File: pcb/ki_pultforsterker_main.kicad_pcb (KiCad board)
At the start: 2 copper layers, 150 x 100 mm, 145 parts, among them J1 24V IN, J10 LED-RINGER, J2 SPK L, J3 SPK R, J4 AUX, J5 RPi 40-pin, J6 5V -> PI, J7 KNAPPER, J8 ENCODER, J9 OLED, K1 G6K-2P-Y 5VDC, Q1 AO3400A, Q2 AO3400A, Q3 AO3400A, Q4 AO3400A, Q5 AO3400A, Q6 AO3400A, U1 TPS54560BDDA, U2 AMS1117-3.3, U3 ICL7660, U4 PCM5102APW, U5 PGA2311UA, U6 TPA3116D2DAD

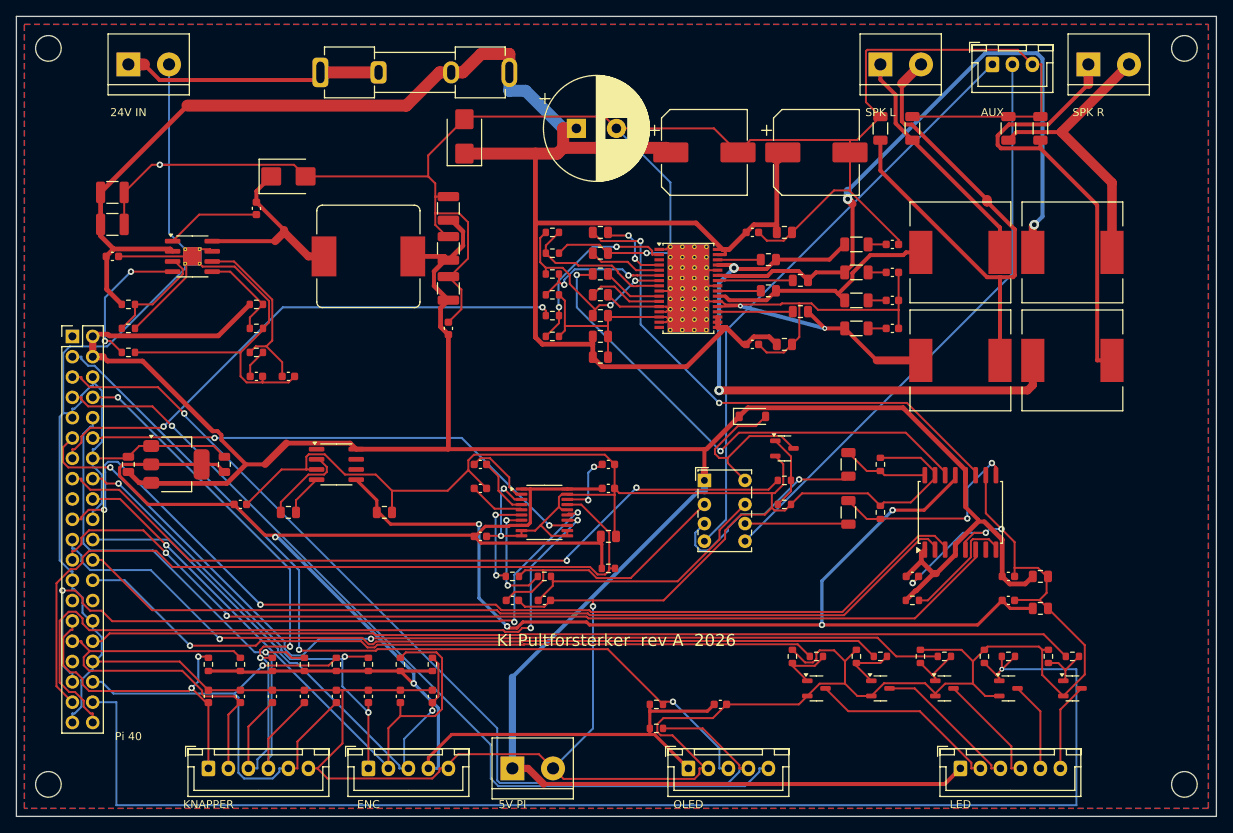
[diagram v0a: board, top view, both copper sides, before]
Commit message: PCB: faste forruter i riktig enhet (µm)
Co-Authored-By: Claude Fable 5.1 <noreply@anthropic.com>
Claude-Session: https://claude.ai/code/session_01FaJKmYinw8SWRobKXBRYpt
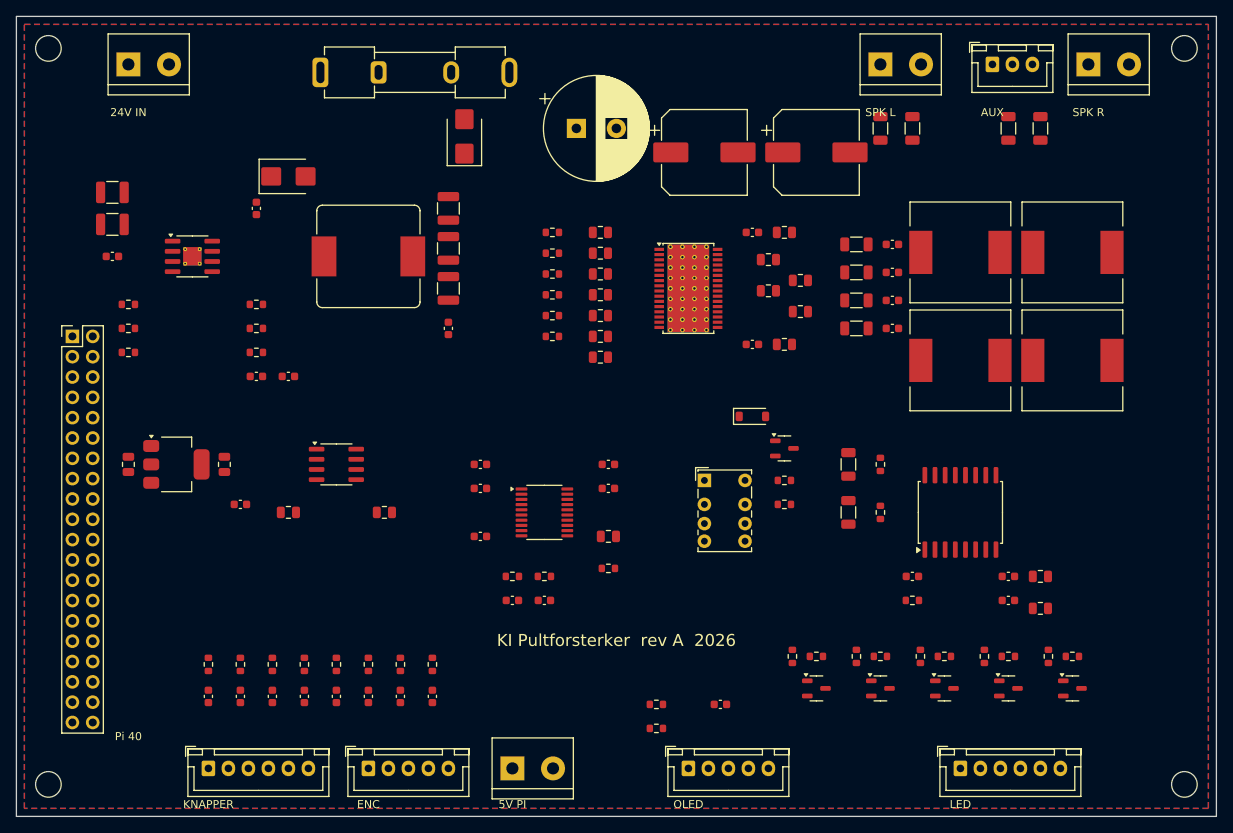
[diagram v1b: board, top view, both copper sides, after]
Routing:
- net GND: track 1090.8 -> 0.00 mm, vias 8 -> 0
- net 5V: track 348.1 -> 0.00 mm
- net VIN24: track 234.9 -> 0.00 mm
- net 3V3: track 222.8 -> 0.00 mm, vias 2 -> 0
- net LED_USB_G: track 163.8 -> 0.00 mm, vias 1 -> 0
- net VNEG: track 128.9 -> 0.00 mm, vias 4 -> 0
- net SPI_MOSI: track 128.2 -> 0.00 mm, vias 2 -> 0
- net LED_AUX_G: track 125.3 -> 0.00 mm, vias 2 -> 0
- net SPI_SCLK: track 124.4 -> 0.00 mm, vias 2 -> 0
- net SCL: track 123.6 -> 0.00 mm, vias 1 -> 0
- net LED_PWR_G: track 123.3 -> 0.00 mm
- net SPI_CS: track 112.9 -> 0.00 mm
- net SDA: track 111.2 -> 0.00 mm, vias 2 -> 0
- net OLED_RES: track 110.9 -> 0.00 mm, vias 1 -> 0
- net LED_BT_G: track 107.8 -> 0.00 mm, vias 1 -> 0
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
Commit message: PCB: OUTPR forrutet fast
Co-Authored-By: Claude Fable 5.1 <noreply@anthropic.com>
Claude-Session: https://claude.ai/code/session_01FaJKmYinw8SWRobKXBRYpt
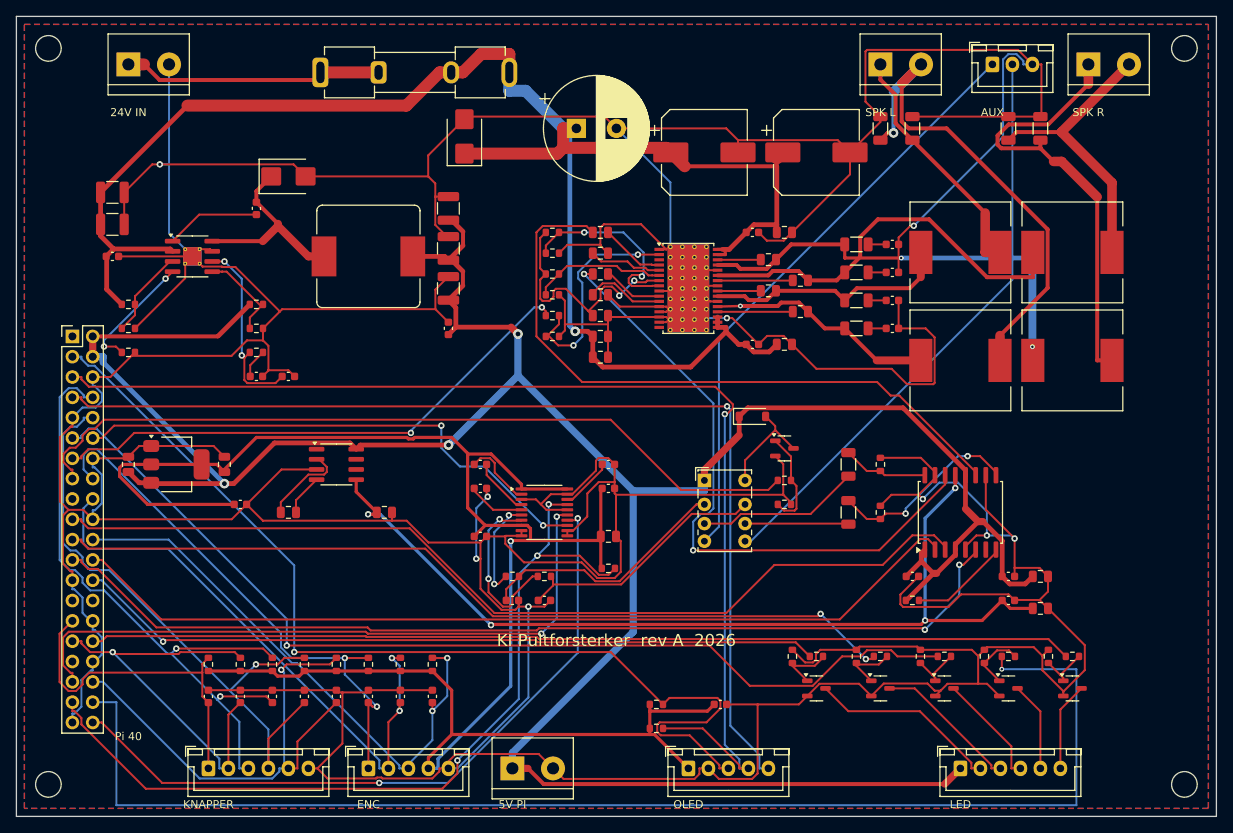
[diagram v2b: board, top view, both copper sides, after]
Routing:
- net GND: track 0.00 -> 1117.5 mm, vias 0 -> 9
- net 5V: track 0.00 -> 350.7 mm, vias 0 -> 3
- net 3V3: track 0.00 -> 238.8 mm, vias 0 -> 1
- net VIN24: track 0.00 -> 221.9 mm, vias 0 -> 1
- net LED_USB_G: track 0.00 -> 163.8 mm, vias 0 -> 1
- net SCL: track 0.00 -> 145.1 mm, vias 0 -> 1
- net OLED_RES: track 0.00 -> 130.5 mm, vias 0 -> 1
- net SDA: track 0.00 -> 127.6 mm, vias 0 -> 1
- net LED_AUX_G: track 0.00 -> 126.3 mm, vias 0 -> 1
- net SPI_SCLK: track 0.00 -> 123.5 mm, vias 0 -> 2
- net LED_PWR_G: track 0.00 -> 122.9 mm
- net SPI_MOSI: track 0.00 -> 119.1 mm
- net VNEG: track 0.00 -> 116.6 mm, vias 0 -> 4
- net SPI_CS: track 0.00 -> 113.3 mm
- net LED_BT_G: track 0.00 -> 106.9 mm, vias 0 -> 2
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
